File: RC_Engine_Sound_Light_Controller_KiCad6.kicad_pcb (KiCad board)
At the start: 2 copper layers, 87 x 39 mm, 42 parts, among them J1 RX, J10 RGB, J11 32, J12 CH1, J13 CH2, J14 CH3, J15 ESC, J16 CH4, J17 Brushed Motor output, J2 HeadL, J3 TailL, J4 RoofL, J5 RevL, J6 Indic, J7 Indic, J8 Battery input, J9 FogL, U1 ESP32_DEVKITV1_30PIN, U2 MP1584EN_BreakoutBoard, U3 PAM8403_BreakoutBoard, U4 ULN2003, U5 RZ7886

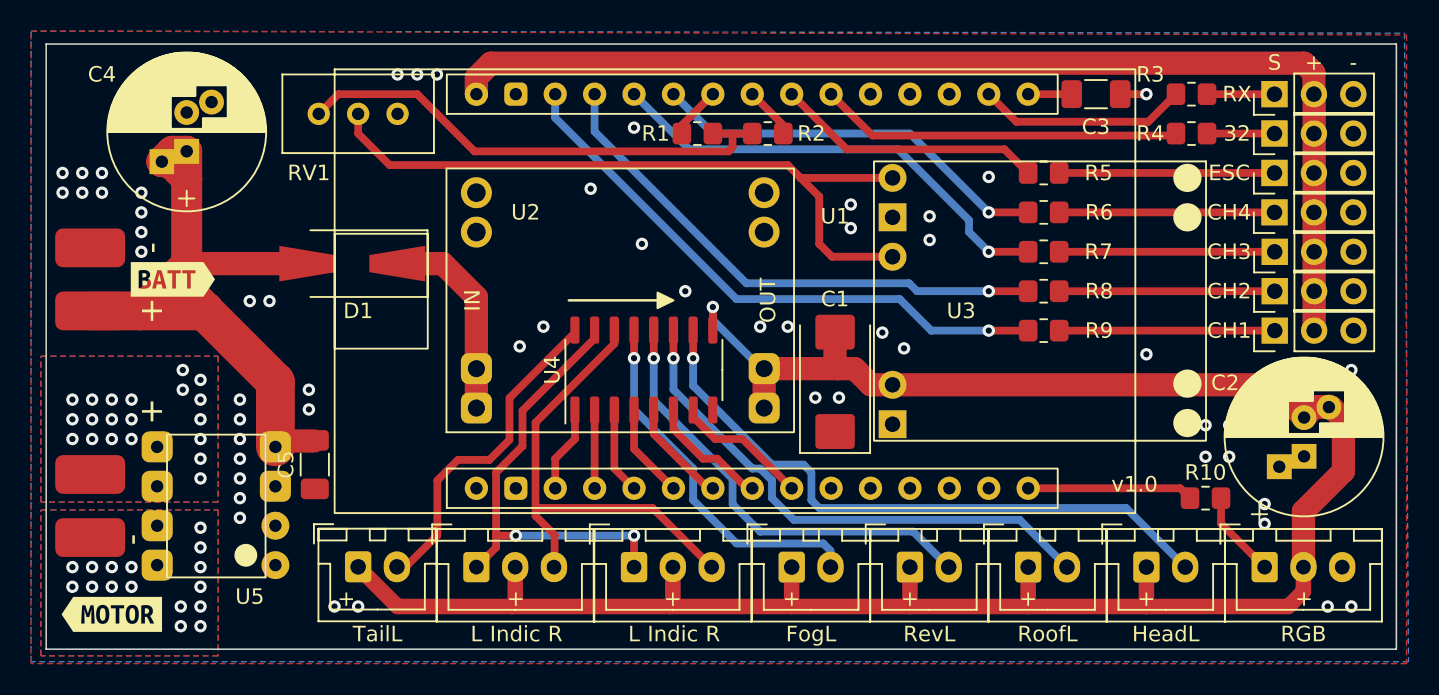
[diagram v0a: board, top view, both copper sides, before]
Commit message: Minor corrections.
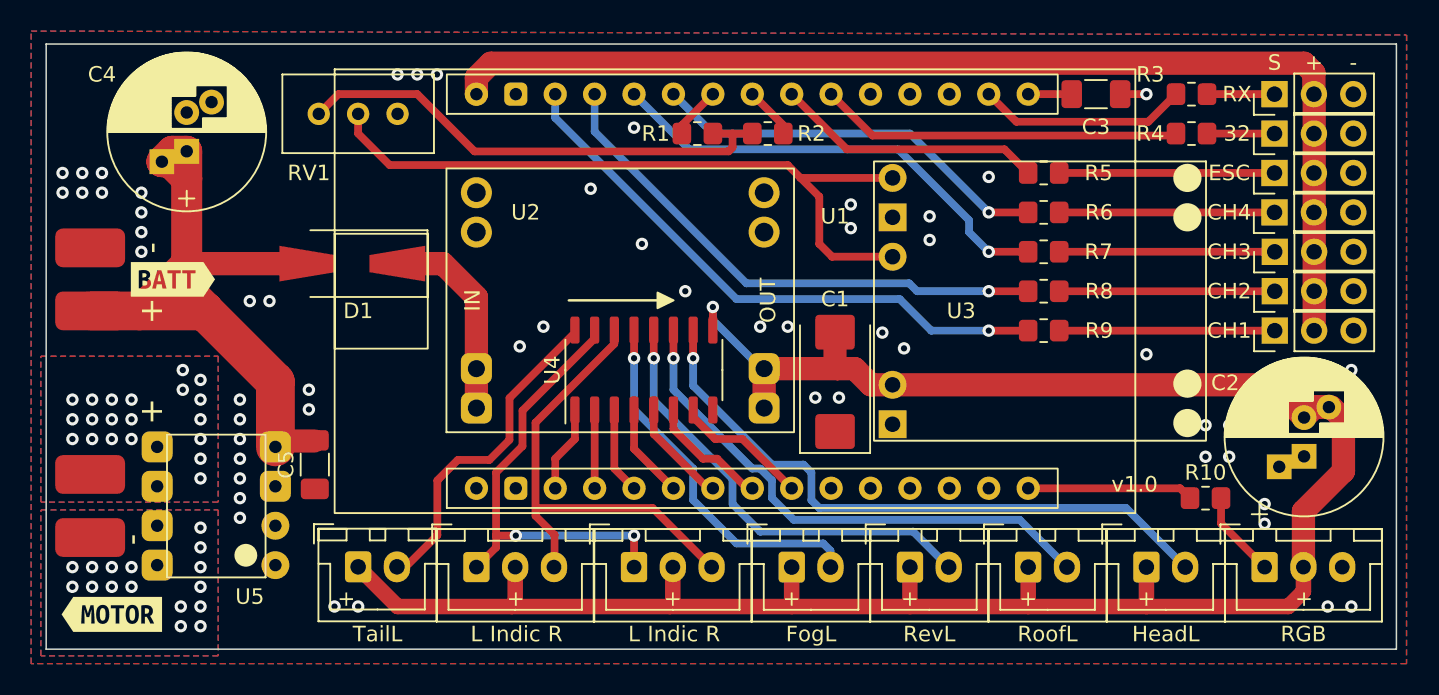
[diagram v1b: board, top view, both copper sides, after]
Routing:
- net /MOTOR_FO: vias 15 -> 20
- net /MOTOR_BO: vias 12 -> 16
- net (no net): vias 9 -> 0
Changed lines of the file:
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@@
       (net 10 "D18") (pinfunction "I7") (pintype "input"))
     (pad "8" smd roundrect (at -2.575 4.445 90) (size 1.75 0.6) (layers "F.Cu" "F.Paste" "F.Mask") (roundrect_rratio 0.25)
-      (net 2 "GND") (pinfunction "GND") (pintype "power_in"))
+      (net 2 "GND") (pinfunction "GND") (pintype "power_in") (zone_connect 2) (thermal_width 0.1) (thermal_gap 0.2))
     (pad "9" smd roundrect (at 2.575 4.445 90) (size 1.75 0.6) (layers "F.Cu" "F.Paste" "F.Mask") (roundrect_rratio 0.25)
       (net 3 "+5V") (pinfunction "COM") (pintype "passive"))
@@
     (effects (font (size 1 1) (thickness 0.15)))
   )
-  (via (at 70.485 71.755) (size 0.8) (drill 0.4) (layers "F.Cu" "B.Cu") (free) (net 0))
-  (via (at 70.485 70.485) (size 0.8) (drill 0.4) (layers "F.Cu" "B.Cu") (free) (net 0))
-  (via (at 73.787 67.31) (size 0.8) (drill 0.4) (layers "F.Cu" "B.Cu") (free) (net 0))
-  (via (at 73.787 68.58) (size 0.8) (drill 0.4) (layers "F.Cu" "B.Cu") (free) (net 0))
-  (via (at 73.66 83.82) (size 0.8) (drill 0.4) (layers "F.Cu" "B.Cu") (free) (net 0))
-  (via (at 73.66 82.55) (size 0.8) (drill 0.4) (layers "F.Cu" "B.Cu") (free) (net 0))
-  (via (at 70.485 80.01) (size 0.8) (drill 0.4) (layers "F.Cu" "B.Cu") (free) (net 0))
-  (via (at 70.485 69.215) (size 0.8) (drill 0.4) (layers "F.Cu" "B.Cu") (free) (net 0))
-  (via (at 70.485 81.28) (size 0.8) (drill 0.4) (layers "F.Cu" "B.Cu") (free) (net 0))
   (segment (start 139.795 52.07) (end 144.145 52.07) (width 0.5) (layer "F.Cu") (net 1))
   (segment (start 134.2013 49.53) (end 135.89 49.53) (width 0.5) (layer "F.Cu") (net 2))
@@
   (segment (start 90.551 60.452) (end 92.71 62.611) (width 1.5) (layer "F.Cu") (net 46))
   (segment (start 92.71 67.22) (end 92.71 69.76) (width 1.5) (layer "F.Cu") (net 46))
+  (via (at 70.485 71.755) (size 0.8) (drill 0.4) (layers "F.Cu" "B.Cu") (free) (net 47))
+  (via (at 70.485 70.485) (size 0.8) (drill 0.4) (layers "F.Cu" "B.Cu") (free) (net 47))
   (via (at 67.945 71.755) (size 0.8) (drill 0.4) (layers "F.Cu" "B.Cu") (free) (net 47))
   (via (at 66.675 69.215) (size 0.8) (drill 0.4) (layers "F.Cu" "B.Cu") (free) (net 47))
+  (via (at 73.787 67.31) (size 0.8) (drill 0.4) (layers "F.Cu" "B.Cu") (free) (net 47))
   (via (at 74.93 71.755) (size 0.8) (drill 0.4) (layers "F.Cu" "B.Cu") (free) (net 47))
   (via (at 74.93 69.215) (size 0.8) (drill 0.4) (layers "F.Cu" "B.Cu") (free) (net 47))
   (via (at 69.215 69.215) (size 0.8) (drill 0.4) (layers "F.Cu" "B.Cu") (free) (net 47))
+  (via (at 73.787 68.58) (size 0.8) (drill 0.4) (layers "F.Cu" "B.Cu") (free) (net 47))
   (via (at 66.675 70.485) (size 0.8) (drill 0.4) (layers "F.Cu" "B.Cu") (free) (net 47))
   (via (at 74.93 73.025) (size 0.8) (drill 0.4) (layers "F.Cu" "B.Cu") (free) (net 47))
@@
   (via (at 69.215 70.485) (size 0.8) (drill 0.4) (layers "F.Cu" "B.Cu") (free) (net 47))
   (via (at 69.215 71.755) (size 0.8) (drill 0.4) (layers "F.Cu" "B.Cu") (free) (net 47))
+  (via (at 70.485 69.215) (size 0.8) (drill 0.4) (layers "F.Cu" "B.Cu") (free) (net 47))
   (via (at 74.93 74.295) (size 0.8) (drill 0.4) (layers "F.Cu" "B.Cu") (free) (net 47))
   (via (at 66.675 81.28) (size 0.8) (drill 0.4) (layers "F.Cu" "B.Cu") (free) (net 48))
   (via (at 74.93 78.74) (size 0.8) (drill 0.4) (layers "F.Cu" "B.Cu") (free) (net 48))
+  (via (at 73.66 83.82) (size 0.8) (drill 0.4) (layers "F.Cu" "B.Cu") (free) (net 48))
   (via (at 67.945 81.28) (size 0.8) (drill 0.4) (layers "F.Cu" "B.Cu") (free) (net 48))
   (via (at 74.93 83.82) (size 0.8) (drill 0.4) (layers "F.Cu" "B.Cu") (free) (net 48))
   (via (at 66.675 80.01) (size 0.8) (drill 0.4) (layers "F.Cu" "B.Cu") (free) (net 48))
   (via (at 74.93 81.28) (size 0.8) (drill 0.4) (layers "F.Cu" "B.Cu") (free) (net 48))
+  (via (at 73.66 82.55) (size 0.8) (drill 0.4) (layers "F.Cu" "B.Cu") (free) (net 48))
   (via (at 74.93 82.55) (size 0.8) (drill 0.4) (layers "F.Cu" "B.Cu") (free) (net 48))
+  (via (at 70.485 80.01) (size 0.8) (drill 0.4) (layers "F.Cu" "B.Cu") (free) (net 48))
   (via (at 74.93 77.47) (size 0.8) (drill 0.4) (layers "F.Cu" "B.Cu") (free) (net 48))
   (via (at 69.215 80.01) (size 0.8) (drill 0.4) (layers "F.Cu" "B.Cu") (free) (net 48))
   (via (at 69.215 81.28) (size 0.8) (drill 0.4) (layers "F.Cu" "B.Cu") (free) (net 48))
   (via (at 67.945 80.01) (size 0.8) (drill 0.4) (layers "F.Cu" "B.Cu") (free) (net 48))
+  (via (at 70.485 81.28) (size 0.8) (drill 0.4) (layers "F.Cu" "B.Cu") (free) (net 48))
   (via (at 74.93 80.01) (size 0.8) (drill 0.4) (layers "F.Cu" "B.Cu") (free) (net 48))
   (segment (start 130.27 64.77) (end 144.16 64.77) (width 0.5) (layer "F.Cu") (net 49))
@@
     )
   )
-  (zone (net 2) (net_name "GND") (layer "F.Cu") (name "GND F") (hatch edge 0.508)
+  (zone (net 2) (net_name "GND") (layers F&B.Cu) (name "GND F") (hatch edge 0.508)
     (connect_pads (clearance 0.5))
     (min_thickness 0.7) (filled_areas_thickness no)
@@
       )
     )
-  )
-  (zone (net 2) (net_name "GND") (layer "B.Cu") (name "GND B") (hatch edge 0.508)
-    (connect_pads (clearance 0.5))
-    (min_thickness 0.7) (filled_areas_thickness no)
-    (fill yes (thermal_gap 0.5) (thermal_bridge_width 0.7) (smoothing fillet) (radius 1))
-    (polygon
-      (pts
-        (xy 152.777626 86.110092)
-        (xy 64.008091 86.105204)
-        (xy 64.009771 45.467401)
-        (xy 152.525306 45.599289)
-      )
-    )
